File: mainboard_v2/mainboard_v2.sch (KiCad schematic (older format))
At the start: 30 parts, among them J1 PWR_IN, J2 CLK_IN, J3 Conn_01x50, SW1 RESET, U1 DS1813, U2 W65C02SxP, U3 74HC21, U4 CY62256-70PC, U5 28C256, X1 ACO-xxxMHz

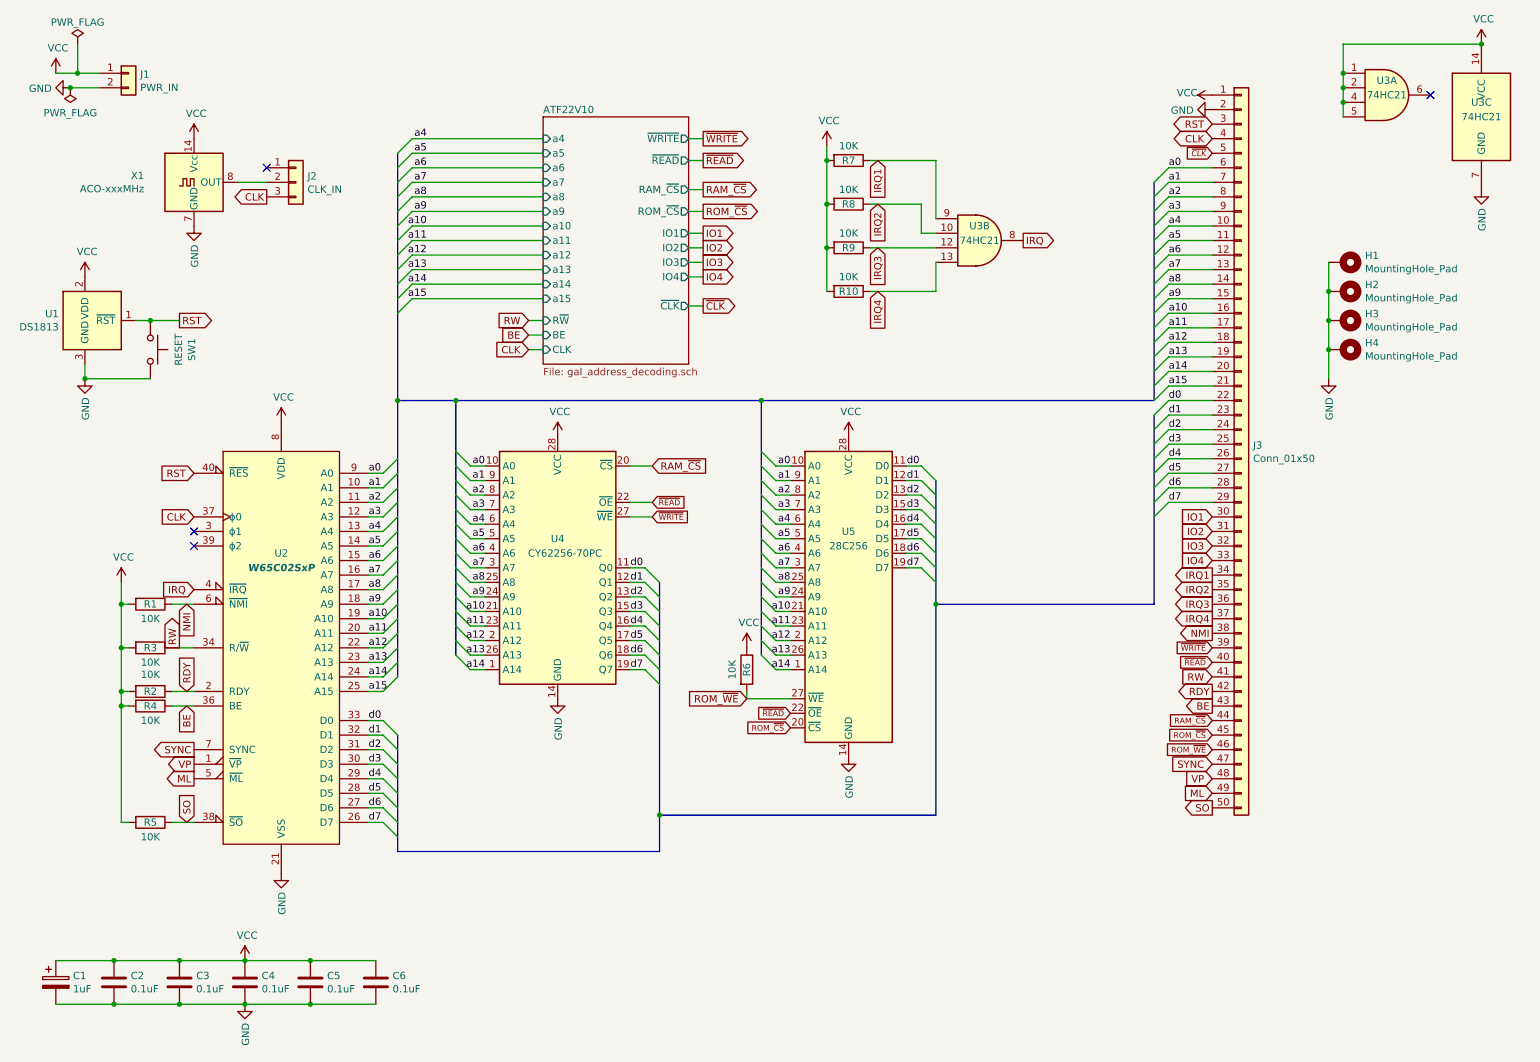
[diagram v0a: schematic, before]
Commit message: Update
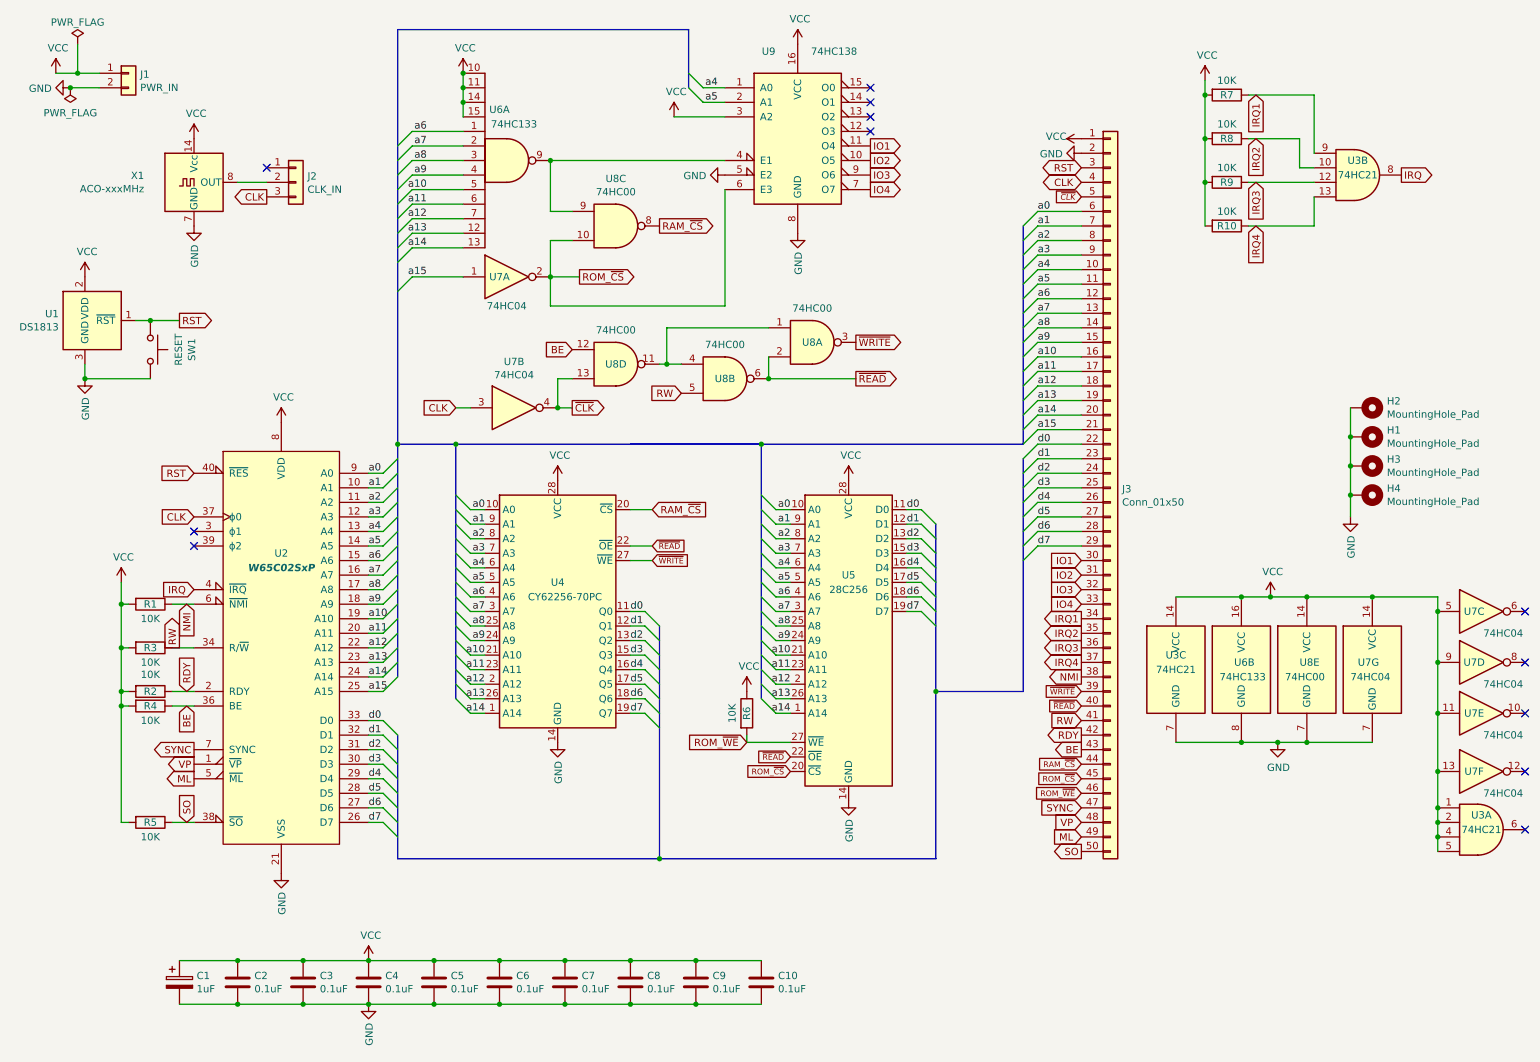
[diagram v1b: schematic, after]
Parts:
- added C10, C7, C8, C9: 0.1uF, Capacitor_THT:C_Disc_D3.0mm_W1.6mm_P2.50mm, symbol Device:C
- added U6: 74HC133, Package_DIP:DIP-16_W7.62mm, symbol 74xx:74LS133
- added U7: 74HC04, Package_DIP:DIP-14_W7.62mm, symbol 74xx:74HC04
- added U8: 74HC00, Package_DIP:DIP-14_W7.62mm, symbol 74xx:74HC00
- added U9: 74HC138, Package_DIP:DIP-16_W7.62mm, symbol 74xx:74LS138
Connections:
- net BE: now also U8.12
- net CLK: now also U7.3
- net GND: now also C10.2, C7.2, C8.2, C9.2, U6.8 (GND), U7.7 (GND), U8.7 (GND), U9.5 (E2), U9.8 (GND)
- net IO1: now also U9.11 (O4)
- net IO2: now also U9.10 (O5)
- net IO3: now also U9.9 (O6)
- net IO4: now also U9.7 (O7)
- net RAM_~CS: now also U8.8
- net ROM_~CS: now also U7.2, U8.10, U9.6 (E3)
- net RW: now also U8.5
- net VCC: now also C10.1, C7.1, C8.1, C9.1, U6.10, U6.11, U6.14, U6.15, U6.16 (VCC), U7.11, U7.13, U7.14 (VCC), U7.5, U7.9, U8.14 (VCC), U9.16 (VCC), U9.3 (A2)
- net a10: now also U6.5
- net a11: now also U6.6
- net a12: now also U6.7
- net a13: now also U6.12
- net a14: now also U6.13
- net a15: now also U7.1
- net a4: now also U9.1 (A0)
- net a5: now also U9.2 (A1)
- net a6: now also U6.1
- net a7: now also U6.2
- net a8: now also U6.3
- net a9: now also U6.4
- net ~CLK: now also U7.4, U8.13
- net ~READ: now also U8.2, U8.6
- net ~WRITE: now also U8.3
- new net: U8.1, U8.11, U8.4
- new net: U6.9, U8.9, U9.4 (E1)
- no-connect marks 4 -> 12
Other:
- moved on the sheet: C1, C2, C3, C4, C5, C6, H1, H2, H3, H4, J3, R10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
